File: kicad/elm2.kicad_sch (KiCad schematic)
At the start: 42 parts, among them IC10 AMS S2570-2, IC51 ITT SAA1094-CH, J1 RJ25, J2 RJ9, Q1 BC546B, Q2 BS107, Q3 BC307, Q4 BS107, Q5 BC546B, Q6 BC546B, Q7 PNP, SW1 SW_Slide_DPDT_horizontal, SW2 SW_Push_3PDT

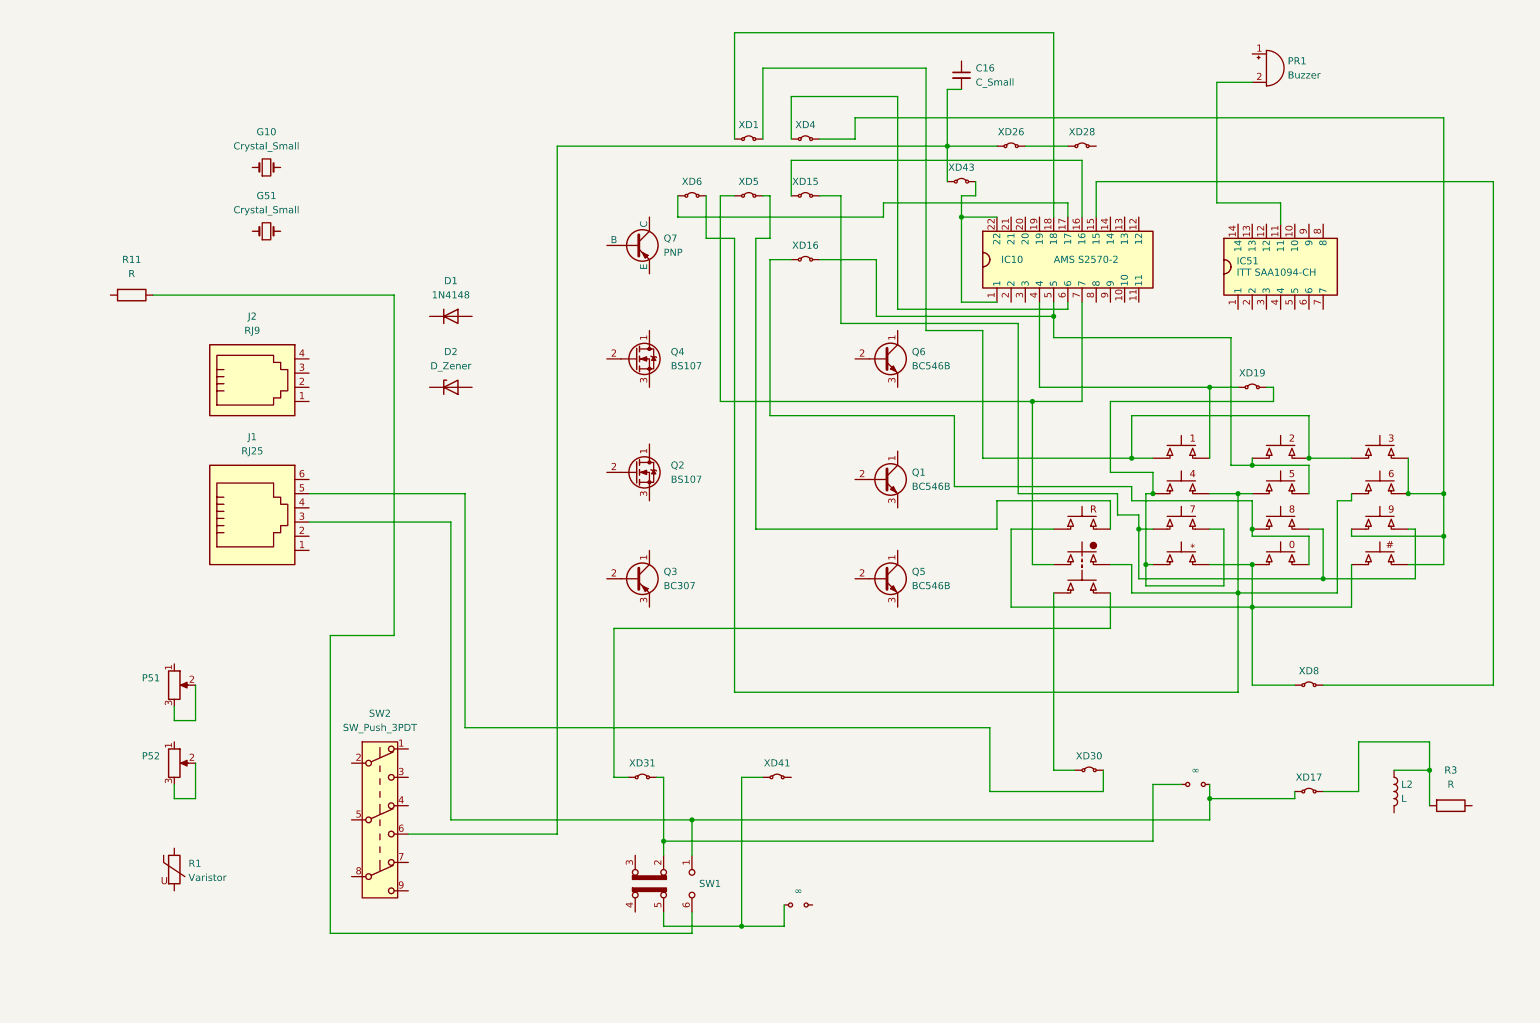
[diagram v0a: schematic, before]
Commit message: Add files via upload
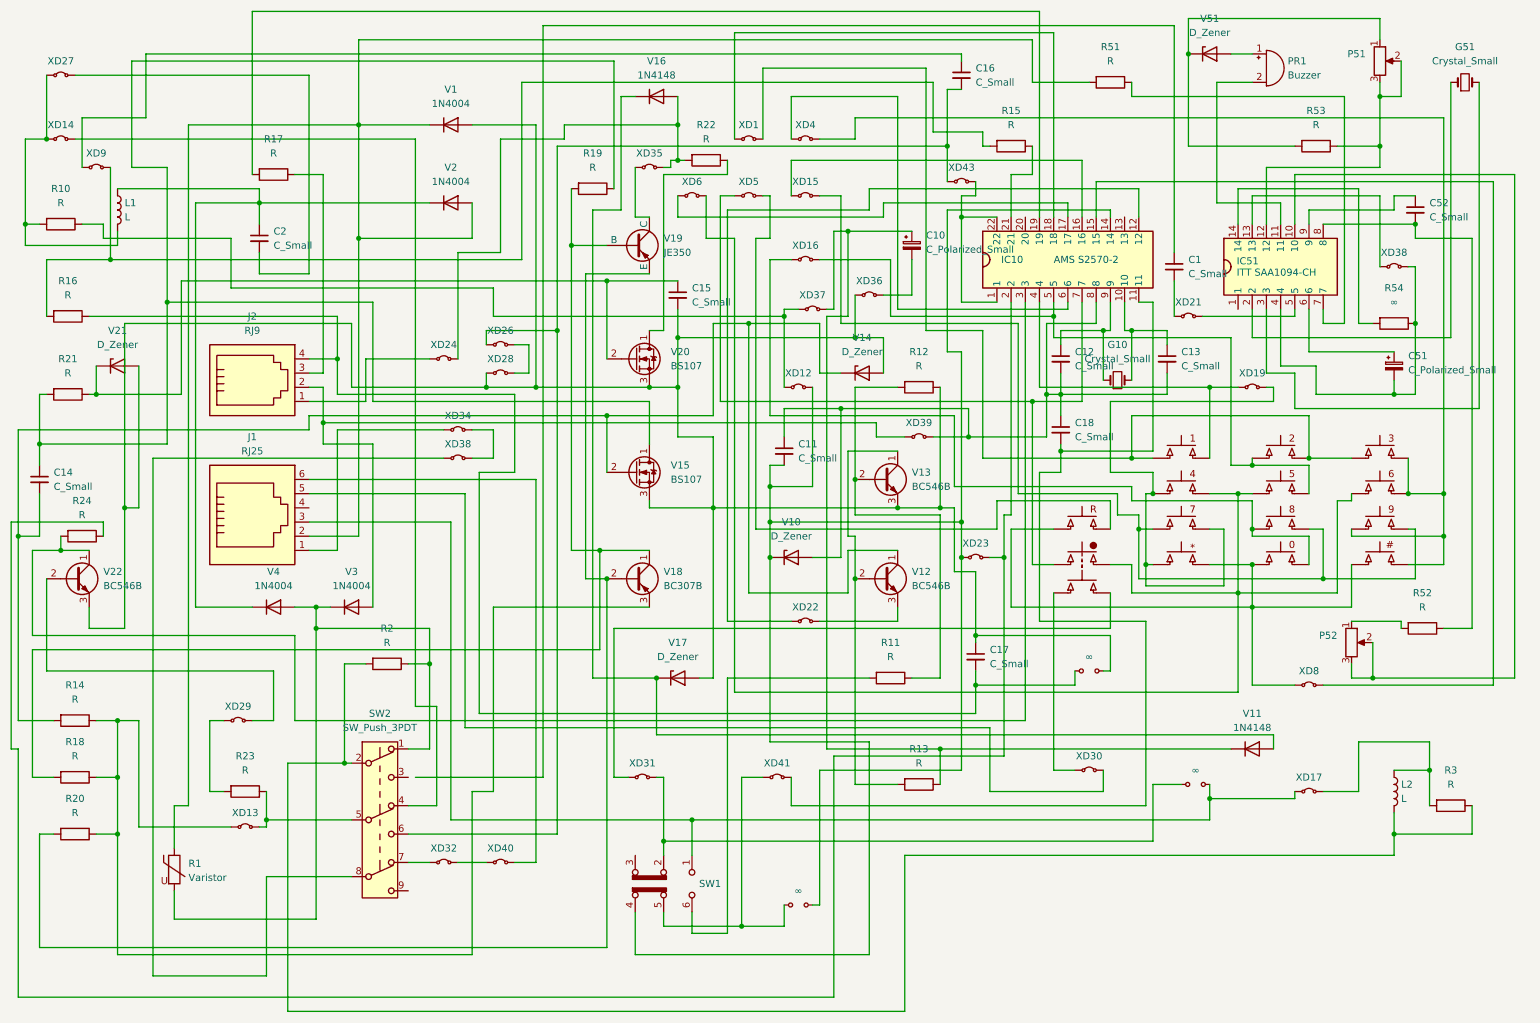
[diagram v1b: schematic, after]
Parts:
- added ?: ∞, symbol Project_Library:R_Unpopulated
- added C1, C11, C12, C13, C14, C15, C17, C18, C2, C52: C_Small, symbol Device:C_Small
- added C10, C51: C_Polarized_Small, symbol Device:C_Polarized_Small
- added L1: L, symbol Device:L
- added R10, R12, R13, R14, R15, R16, R17, R18, R19, R2, R20, R21, R22, R23, R24, R51, R52, R53: R, symbol Device:R
- added R54: ∞, symbol Device:R
- added V1, V2, V3, V4: 1N4004, Diode_THT:D_DO-41_SOD81_P10.16mm_Horizontal, symbol Diode:1N4004
- added V11: 1N4148, Diode_THT:D_DO-35_SOD27_P7.62mm_Horizontal, symbol Diode:1N4148
- added V14, V17, V21, V51: D_Zener, symbol Device:D_Zener
- added XD12, XD13, XD14, XD21, XD22, XD23, XD24, XD27, XD29, XD32, XD34, XD35, XD36, XD37, XD38 (x2), XD39, XD40, XD9: ~, symbol Project_Library:Jumper_2_Small_Bridged
- V18: renamed from Q3; value BC307 -> BC307B
- V19: renamed from Q7; value PNP -> JE350
- renumbered D2 to V10, Q5 to V12, Q1 to V13, Q2 to V15, D1 to V16, Q4 to V20, Q6 to V22
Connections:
- net at XD28.1 (A): now also ?.1, V13.3 (E), V15.3 (S), V20.3 (S), V22.3 (E), C15.2, C17.1, R12.1, V1.2 (A), V14.2 (A), V17.2 (A), V21.2 (A), XD36.1 (A); no longer XD26.2 (B)
- net at XD28.2 (B): now also XD26.2 (B)
- net at V18.1 (C): now also V19.2 (B), R18.2, R19.2
- net at V18.2 (B): now also V19.3 (E), R20.2
- net at V18.3 (E): now also R14.1, R18.1, R20.1, XD13.1 (A)
- net at V20.1 (D): now also R22.1
- net at V20.2 (G): now also C15.1, R21.1, V21.1 (K)
- net at IC51.10: now also P52.2, P52.3
- net at IC51.12: now also P51.2, P51.3, R53.1
- net at IC51.13: now also XD38.1 (A)
- net at IC51.14: now also R54.2
- net at IC51.2: now also G51.1
- net at IC51.3: now also G51.2
- net at IC51.4: now also C51.2, R54.1, XD38.2 (B)
- net at IC51.5: now also XD21.2 (B)
- net at IC51.6: now also C51.1
- net at IC51.7: now also R51.1
- net at IC51.8: now also C52.2, R52.1
- net at IC51.9: now also C52.1
- net at V13.1 (C): now also V12.2 (B), R13.2
- net at V13.2 (B): now also R11.1, R12.2
- net at IC10.10: now also G10.2, C13.1
- net at IC10.11: now also XD41.2 (B), C18.2
- net at IC10.12: now also XD22.1 (A)
- net at IC10.14: now also SW1.4 (A), V10.1 (K), ?.1, C11.2, XD12.2 (B), XD23.1 (A)
- net at IC10.19: now also R17.2
- net at IC10.2: now also R24.1, XD23.2 (B)
- net at IC10.21: now also R15.1
- net at IC10.3: now also V22.1 (C), R24.2
- net at IC10.8: now also V10.2 (A), C11.1, C12.2, C13.2, C18.1, XD39.2 (B)
- net at IC10.9: now also G10.1, C12.1
- net at KEYPAD1.3 (B), KEYPAD1.4 (B): now also XD31.1 (A); no longer XD5.2 (B)
- net at SW2.1 (A): now also R1.2, R2.1, V3.1 (K), V4.2 (A)
- net at SW2.2 (B): now also L2.2, R3.1, R2.2
- net at SW2.4 (A): now also XD14.2 (B)
- net at SW2.5 (B): now also R23.1, XD13.2 (B)
- net at SW2.7 (A): now also XD32.1 (A)
- net at SW2.8 (B): now also XD38.1 (A)
- net at V22.2 (B): now also XD29.2 (B)
- net at PR1.1 (+): now also V51.2 (A)
- net at P52.1: now also R52.2
- net at V12.1 (C): now also V15.2 (G), C14.2, R14.2, V14.1 (K)
- net at V12.3 (E): now also XD22.2 (B)
- net at P51.1: now also R53.2, V51.1 (K)
- net at V16.1 (K): now also V11.2 (A), V17.1 (K)
- net at V16.2 (A): now also R22.2, XD24.2 (B), XD35.2 (B)
- net at SW1.6 (C): now also R11.2; no longer R11.1
- net at C16.1: now also XD9.1 (A)
- net at SW1.5 (B), XD41.1 (A): now also ?.2; no longer ?.2
- net at V19.1 (C): now also XD35.1 (A)
- net at R1.1: now also J1.2, R51.2, V1.1 (K), V2.2 (A)
- net at J1.1: now also XD34.1 (A)
- net at J1.6: now also XD40.2 (B)
- net at J2.1: now also XD24.1 (A)
- net at J2.2: now also V3.2 (A), XD39.1 (A)
- net at J2.3: now also R17.1
- net at J2.4: now also ?.2, C17.2, R16.1
- net at V15.1 (D): now also C14.1, R19.1, R21.2
- new net: R10.1, XD12.1 (A), XD37.1 (A)
- new net: C10.1, R13.1, V11.1 (K), XD37.2 (B)
- new net: XD34.2 (B), XD38.2 (B)
- new net: KEYPAD1.1 (A), KEYPAD1.2 (A), KEYPAD1.3 (B), KEYPAD1.4 (B), XD8.1 (A)
- new net: KEYPAD1.1 (A), KEYPAD1.2 (A), KEYPAD1.3 (B), KEYPAD1.4 (B), XD16.1 (A)
- new net: IC10.5, KEYPAD1.1 (A), KEYPAD1.2 (A), KEYPAD1.3 (B), KEYPAD1.4 (B), XD16.2 (B)
- new net: R23.2, XD29.1 (A)
- new net: C10.2, XD36.2 (B)
- new net: C2.1, L1.1, V2.1 (K), V4.1 (K)
- new net: L1.2, R10.2, XD14.1 (A), XD27.1 (A)
- new net: C1.2, XD21.1 (A)
- new net: KEYPAD1.1 (A), KEYPAD1.2 (A), KEYPAD1.3 (B), KEYPAD1.4 (B), XD1.2 (B)
- new net: XD32.2 (B), XD40.1 (A)
- new net: KEYPAD1.1 (A), KEYPAD1.2 (A), KEYPAD1.3 (B), KEYPAD1.4 (B), XD6.2 (B)
- new net: KEYPAD1.1 (A), KEYPAD1.2 (A), KEYPAD1.3 (B), KEYPAD1.4 (B), XD15.2 (B)
- new net: KEYPAD1.1 (A), KEYPAD1.2 (A), KEYPAD1.3 (B), KEYPAD1.4 (B), XD4.2 (B)
- new net: KEYPAD1.1 (A), KEYPAD1.2 (A), KEYPAD1.3 (B), KEYPAD1.4 (B), XD19.2 (B)
- new net: KEYPAD1.3 (B), KEYPAD1.4 (B), XD5.2 (B)
- new net: C2.2, XD27.2 (B)
- new net: R15.2, R16.2, XD9.2 (B)
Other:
- moved on the sheet: G10, G51, P51, P52, V10, V16, V22

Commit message: Add files via upload
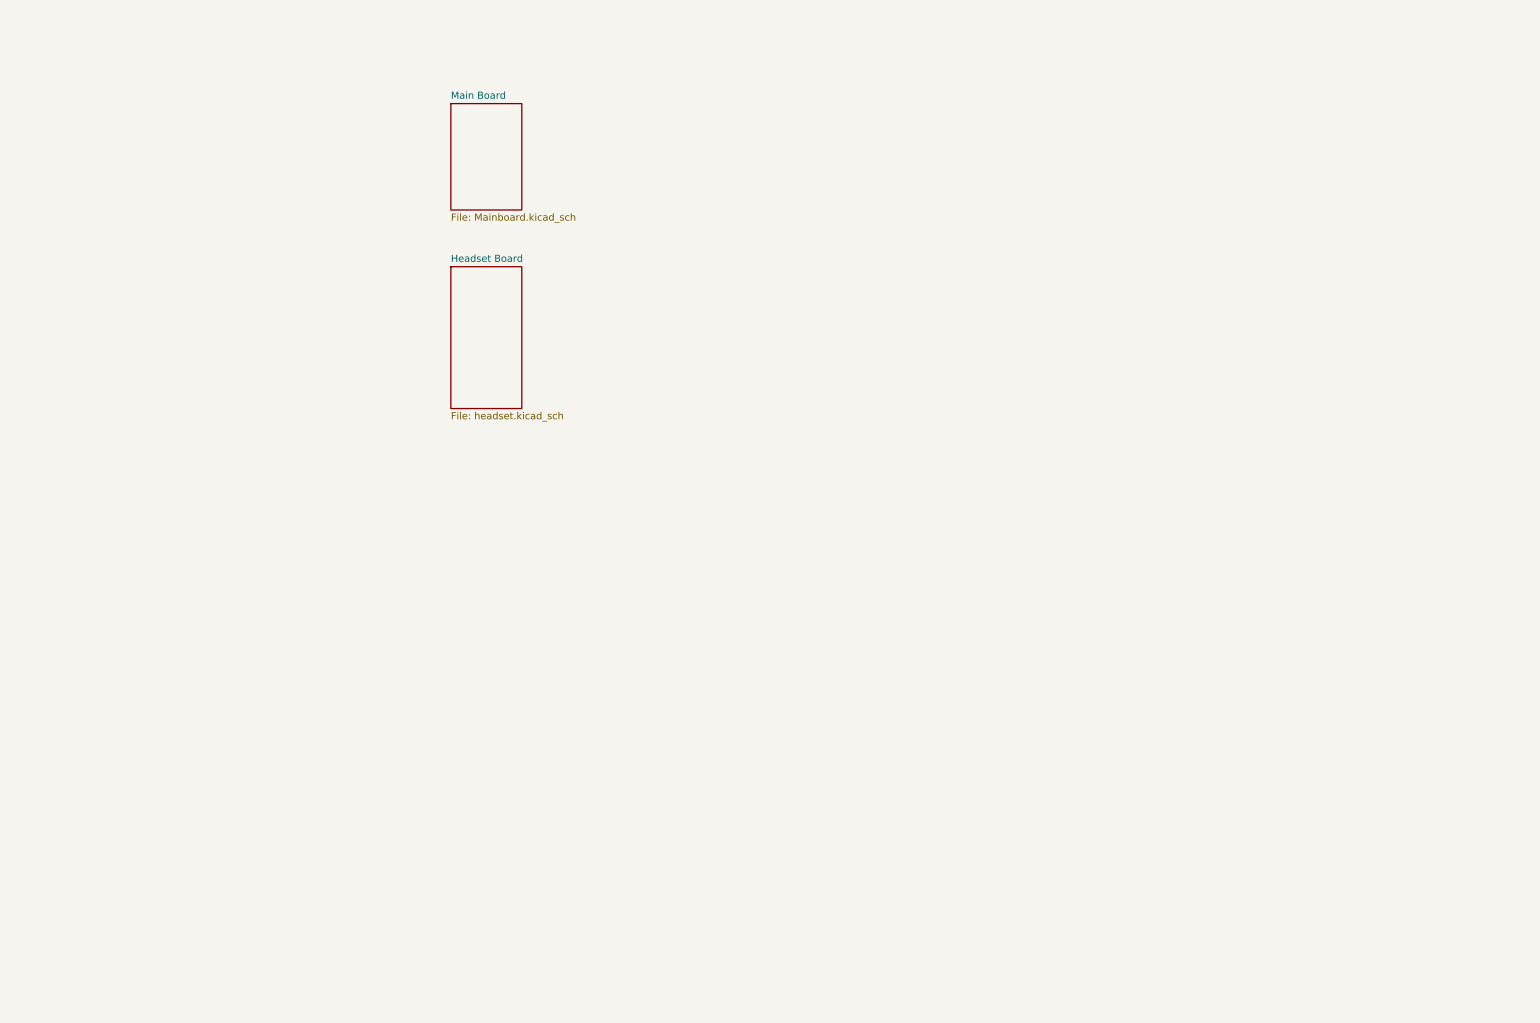
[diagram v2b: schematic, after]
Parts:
- removed ? (x2): ∞, symbol Project_Library:R_Unpopulated
- removed C1, C11, C12, C13, C14, C15, C16, C17, C18, C2, C52: C_Small, symbol Device:C_Small
- removed C10, C51: C_Polarized_Small, symbol Device:C_Polarized_Small
- removed G10, G51: Crystal_Small, symbol Device:Crystal_Small
- removed IC10: AMS S2570-2, symbol Project_Library:S2570-2_DIP22
- removed IC51: ITT SAA1094-CH, symbol Project_Library:SAA1094-CH_DIP14
- removed J1: RJ25, symbol Connector:RJ25
- removed J2: RJ9, symbol Connector:RJ9
- removed KEYPAD1: SW_KEYPAD_PHONE_ELM2, symbol Project_Library:SW_KEYPAD_PHONE_ELM2
- removed L1, L2: L, symbol Device:L
- removed P51, P52: ~, symbol Device:R_Potentiometer
- removed PR1: Buzzer, symbol Device:Buzzer
- removed R1: Varistor, symbol Device:Varistor
- removed R10, R11, R12, R13, R14, R15, R16, R17, R18, R19, R2, R20, R21, R22, R23, R24, R3, R51, R52, R53: R, symbol Device:R
- removed R54: ∞, symbol Device:R
- removed SW1: SW_Slide_DPDT_horizontal, symbol Project_Library:SW_Slide_DPDT_horizontal
- removed SW2: SW_Push_3PDT, symbol Project_Library:SW_Push_3PDT
- removed V1, V2, V3, V4: 1N4004, Diode_THT:D_DO-41_SOD81_P10.16mm_Horizontal, symbol Diode:1N4004
- removed V10, V14, V17, V21, V51: D_Zener, symbol Device:D_Zener
- removed V11, V16: 1N4148, Diode_THT:D_DO-35_SOD27_P7.62mm_Horizontal, symbol Diode:1N4148
- removed V12, V13, V22: BC546B, Package_TO_SOT_THT:TO-92_Inline, symbol Transistor_BJT:BC546
- removed V15, V20: BS107, Package_TO_SOT_THT:TO-92_Inline, symbol Transistor_FET:BS107
- removed V18: BC307B, Package_TO_SOT_THT:TO-92_Inline, symbol Transistor_BJT:BC307
- removed V19: JE350, symbol Simulation_SPICE:PNP
- removed XD1, XD12, XD13, XD14, XD15, XD16, XD17, XD19, XD21, XD22, XD23, XD24, XD26, XD27, XD28, XD29, XD30, XD31, XD32, XD34, XD35, XD36, XD37, XD38 (x2), XD39, XD4, XD40, XD41, XD43, XD5, XD6, XD8, XD9: ~, symbol Project_Library:Jumper_2_Small_Bridged
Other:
- added sheet Headset Board (headset.kicad_sch)
- added sheet Main Board (Mainboard.kicad_sch)
